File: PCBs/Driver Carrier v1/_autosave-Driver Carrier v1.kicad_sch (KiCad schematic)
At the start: 12 parts, among them J10 Limit Switch Connector n4, J11 Limit Switch Connector n5, J12 Limit Switch Connector n6, J13 CAN Connector, J14 Screw_Terminal_01x02, J15 Screw_Terminal_01x02, J16 Controller Reset, J17 Remaining GPIOs, J7 Limit Switch Connector n1, J8 Limit Switch Connector n2, J9 Limit Switch Connector n3, U13 ESP32-S3-DEVKITM

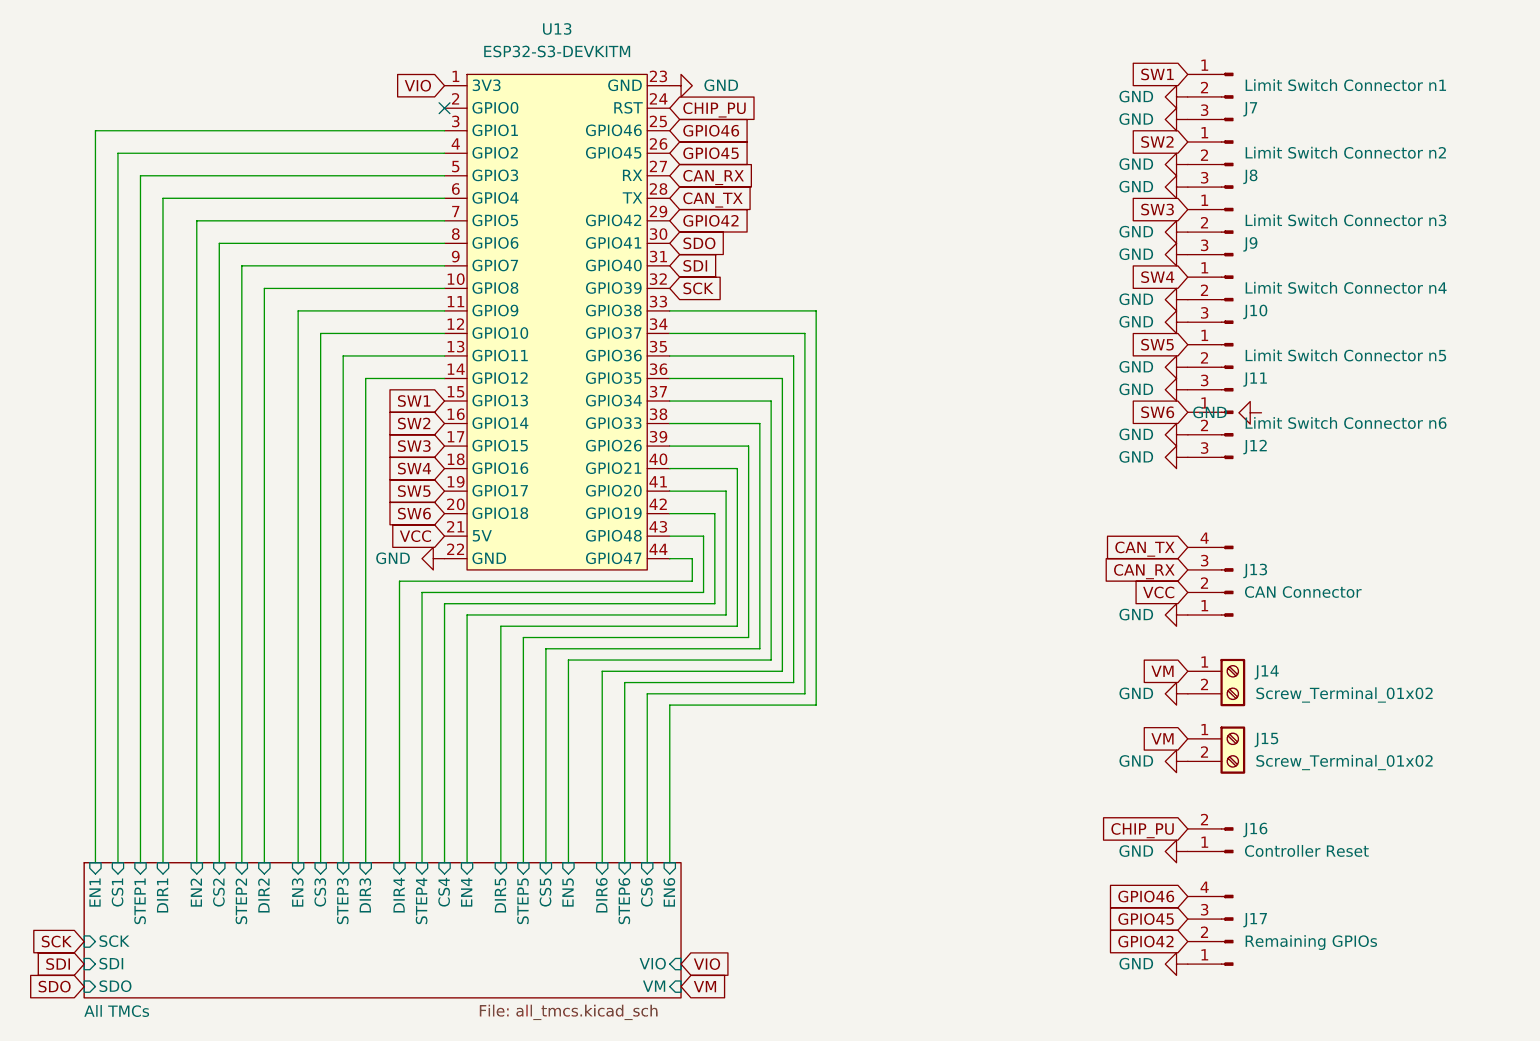
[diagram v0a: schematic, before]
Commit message: Finished Driver Carrier
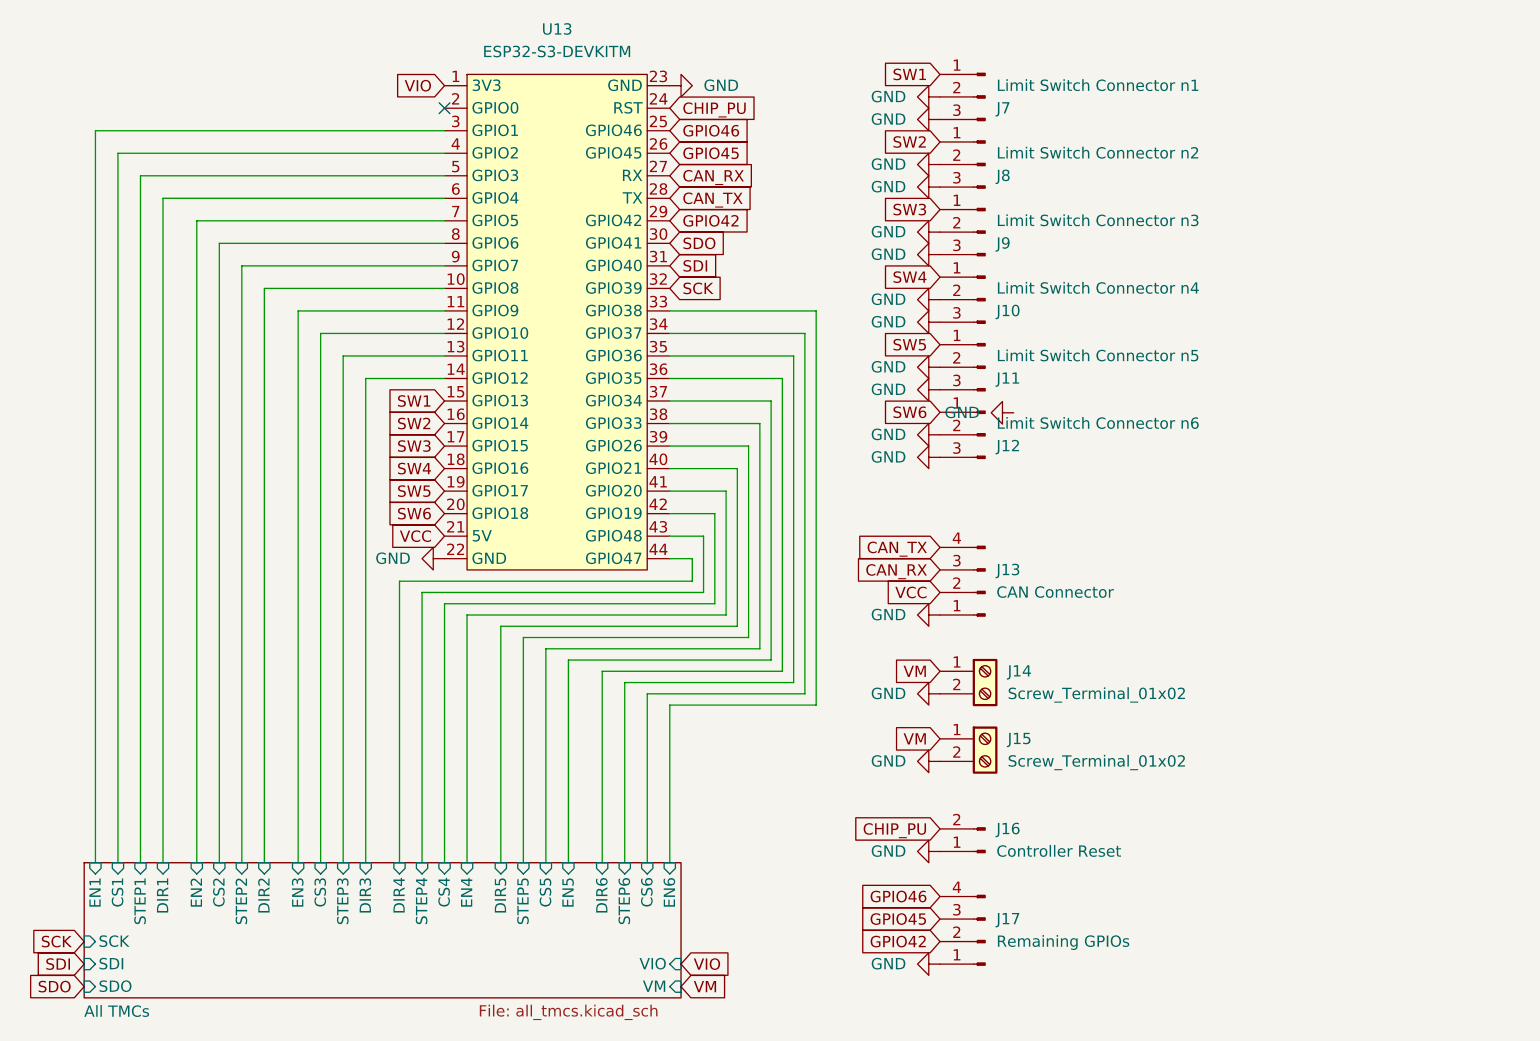
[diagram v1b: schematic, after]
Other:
- moved on the sheet: J10, J11, J12, J13, J14, J15, J16, J17, J7, J8, J9
